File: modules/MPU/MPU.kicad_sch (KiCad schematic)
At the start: 6 parts, among them J1 CardConnector, U1 74HCT541, U2 74HCT00

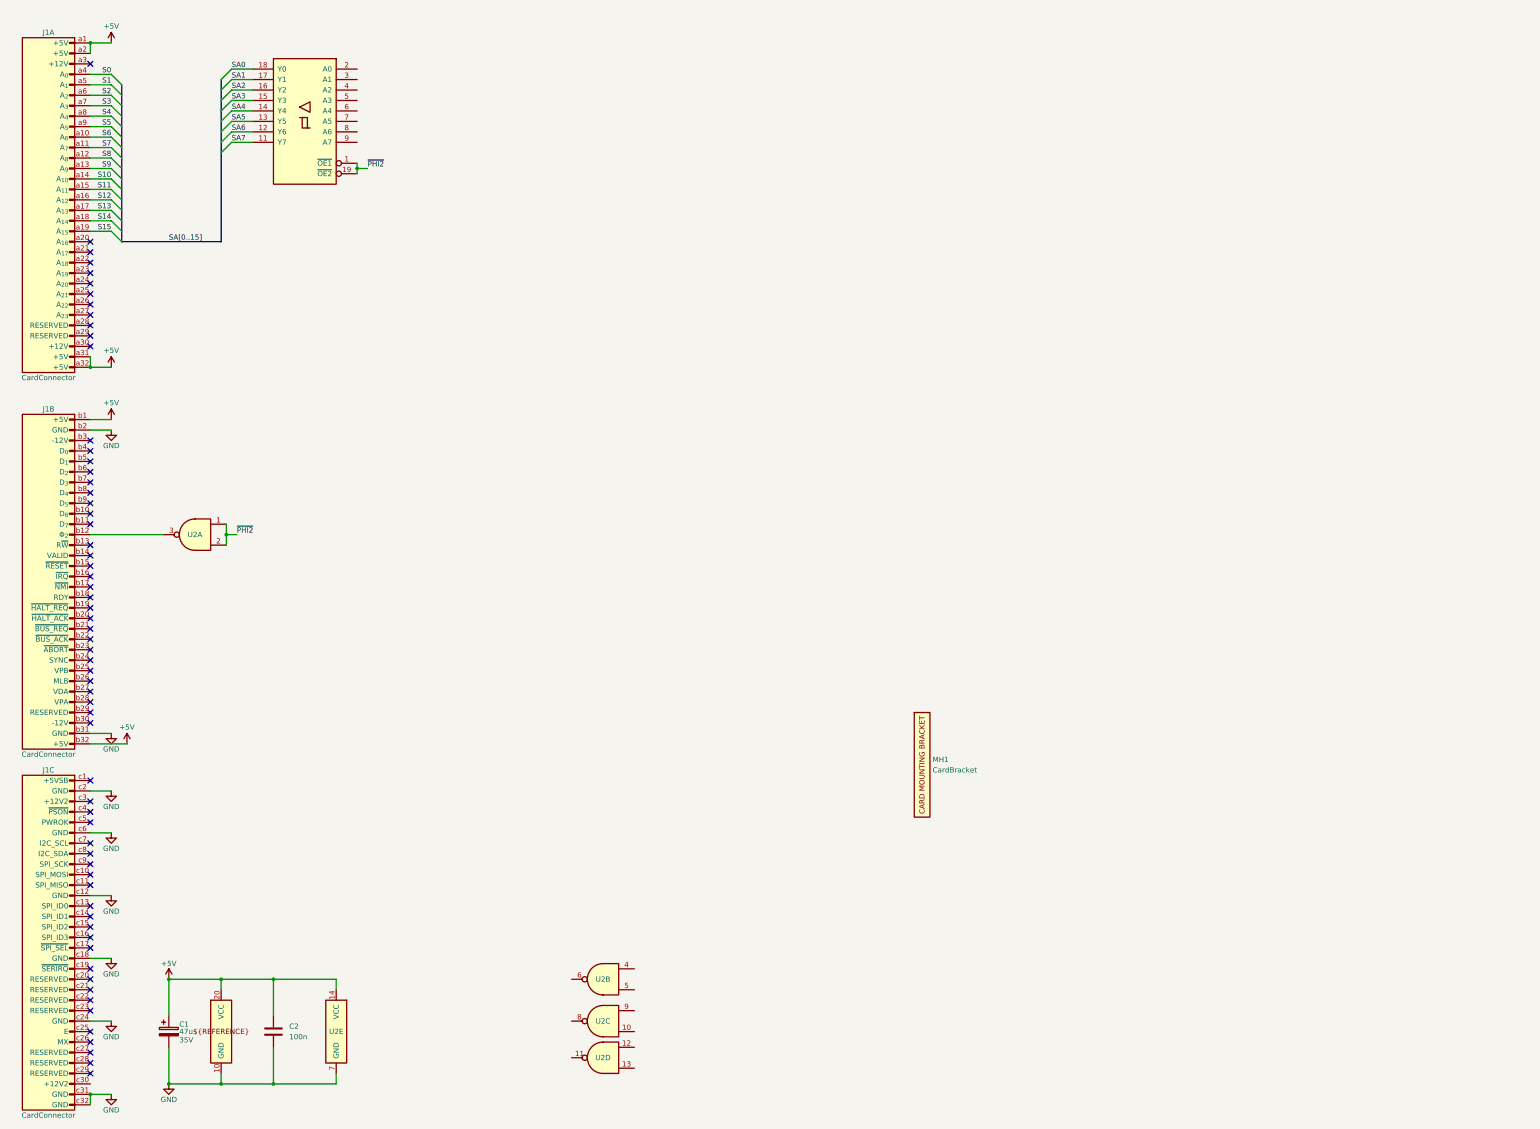
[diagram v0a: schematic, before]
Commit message: mpu wip
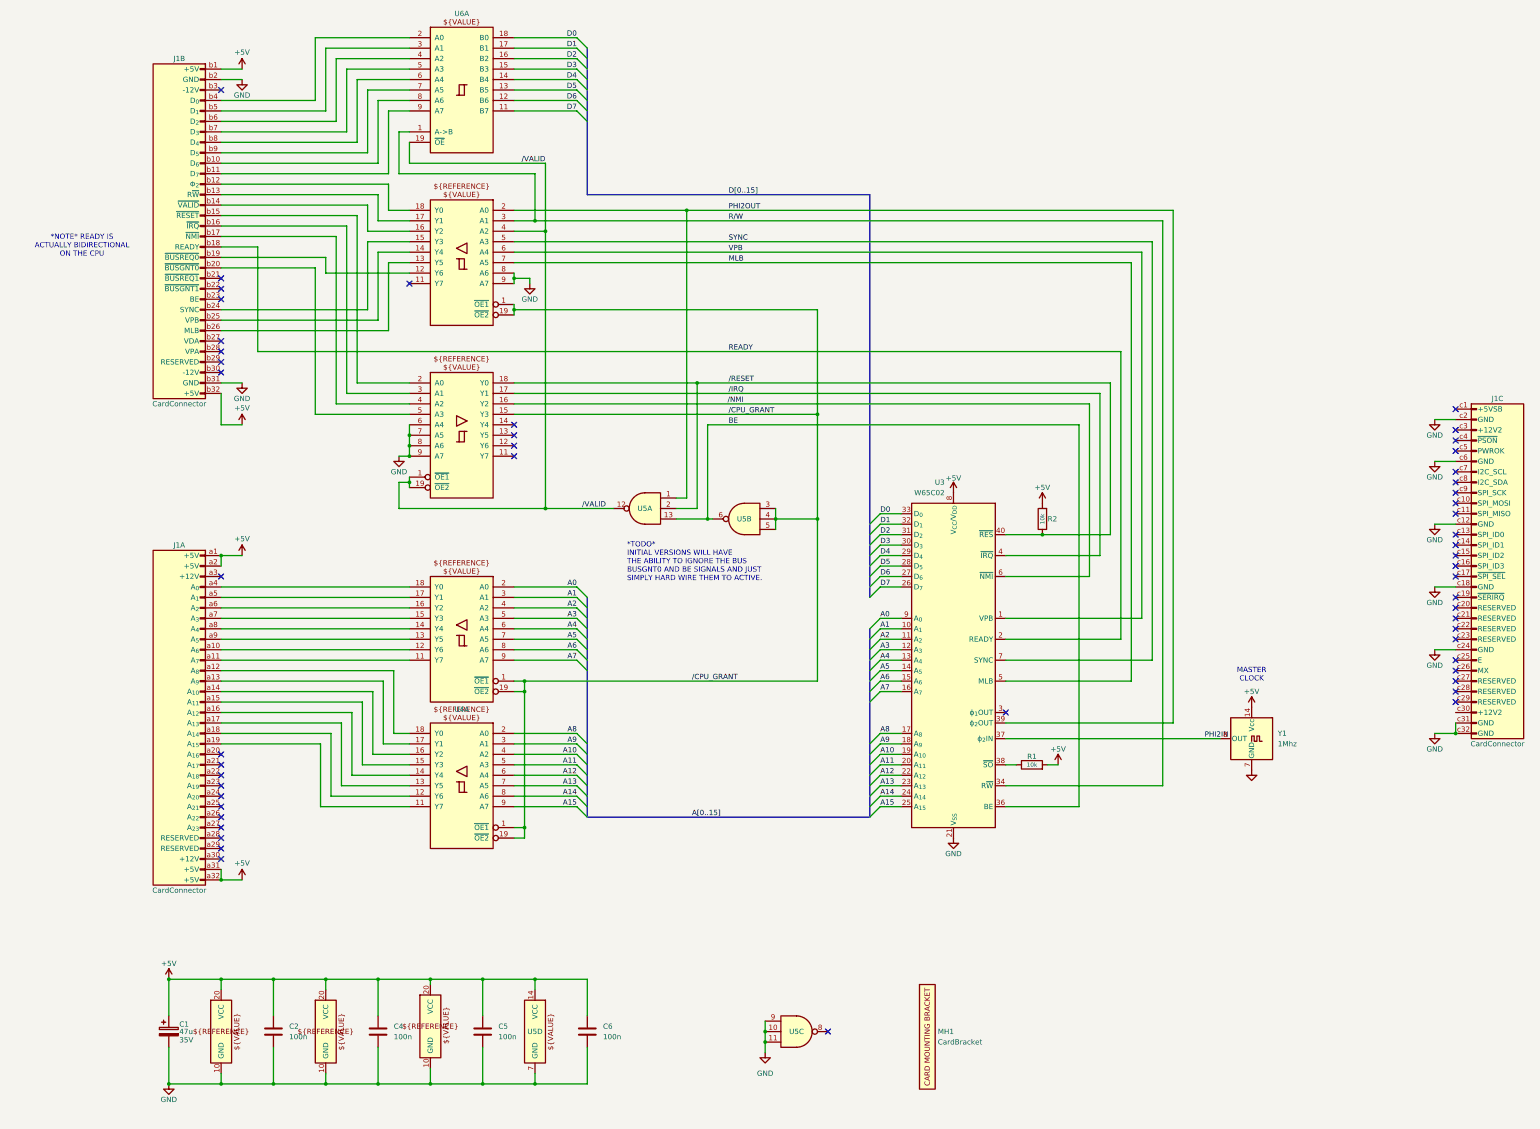
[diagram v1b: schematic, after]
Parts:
- removed U2: 74HCT00, IMNOTWOPR:DIP-14N, symbol IMNOTWOPR:74HCT00
- added C4, C5, C6: 100n, FormantKO:C_Rect_P200mil, symbol FormantKO:C
- added R1, R2: 10k, IMNOTWOPR:R_Axial_DIN0207_P400mil, symbol IMNOTWOPR:R
- added unit 1 of U1
- added U3: W65C02, IMNOTWOPR:DIP-40W, symbol IMNOTWOPR:W65C02
- added U4, U7, U8: 74HCT541, IMNOTWOPR:DIP-20N, symbol IMNOTWOPR:74HCT541
- added U5: 74HCT10, symbol IMNOTWOPR:74HCT10
- added U6: 74HCT245N, IMNOTWOPR:DIP-20N, symbol IMNOTWOPR:74HCT245
- added Y1: 1Mhz, Oscillator:Oscillator_DIP-14, symbol Oscillator:ACO-xxxMHz
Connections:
- net +5V: now also C4.1, C5.1, C6.1, R1.2, R2.2, U3.8 (V_{CC}/V_{DD}), U4.20 (VCC), U5.14 (VCC), U6.20 (VCC), Y1.14 (Vcc)
- net GND: now also C4.2, C5.2, C6.2, U3.21 (V_{SS}), U4.10 (GND), U5.10, U5.11, U5.7 (GND), U5.9, U6.10 (GND), U7.8 (A6), U7.9 (A7), U8.6 (A4), U8.7 (A5), U8.8 (A6), U8.9 (A7), Y1.7 (GND)
- net at J1.b12 (Φ_{2}): now also U7.18 (Y0)
- net at J1.b10 (D_{6}): now also U6.8 (A6)
- net at J1.b11 (D_{7}): now also U6.9 (A7)
- net at J1.b13 (R~{W}): now also U7.17 (Y1)
- net at J1.b14 (~{VALID}): now also U7.16 (Y2)
- net at J1.b15 (~{RESET}): now also U8.2 (A0)
- net at J1.b16 (~{IRQ}): now also U8.3 (A1)
- net at J1.b17 (~{NMI}): now also U8.4 (A2)
- net READY: now reaches J1.b18 (READY)
- net READY: now also U3.2 (READY)
- net at J1.b19 (~{BUSREQ0}): now also U7.12 (Y6)
- net at J1.b20 (~{BUSGNT0}): now also U8.5 (A3)
- net at J1.b24 (SYNC): now also U7.15 (Y3)
- net at J1.b25 (VPB): now also U7.14 (Y4)
- net at J1.b26 (MLB): now also U7.13 (Y5)
- net at J1.b4 (D_{0}): now also U6.2 (A0)
- net at J1.b5 (D_{1}): now also U6.3 (A1)
- net at J1.b6 (D_{2}): now also U6.4 (A2)
- net at J1.b7 (D_{3}): now also U6.5 (A3)
- net at J1.b8 (D_{4}): now also U6.6 (A4)
- net at J1.b9 (D_{5}): now also U6.7 (A5)
- net S0: no longer names the net of J1.a4 (A_{0})
- net S0: now also U1.18 (Y0)
- net S1: no longer names the net of J1.a5 (A_{1})
- net S1: now also U1.17 (Y1)
- net S10: no longer names the net of J1.a14 (A_{10})
- net S10: now also U4.16 (Y2)
- net S11: no longer names the net of J1.a15 (A_{11})
- net S11: now also U4.15 (Y3)
- net S12: no longer names the net of J1.a16 (A_{12})
- net S12: now also U4.14 (Y4)
- net S13: no longer names the net of J1.a17 (A_{13})
- net S13: now also U4.13 (Y5)
- net S14: no longer names the net of J1.a18 (A_{14})
- net S14: now also U4.12 (Y6)
- net S15: no longer names the net of J1.a19 (A_{15})
- net S15: now also U4.11 (Y7)
- net S2: no longer names the net of J1.a6 (A_{2})
- net S2: now also U1.16 (Y2)
- net S3: no longer names the net of J1.a7 (A_{3})
- net S3: now also U1.15 (Y3)
- net S4: no longer names the net of J1.a8 (A_{4})
- net S4: now also U1.14 (Y4)
- net S5: no longer names the net of J1.a9 (A_{5})
- net S5: now also U1.13 (Y5)
- net S6: no longer names the net of J1.a10 (A_{6})
- net S6: now also U1.12 (Y6)
- net S7: no longer names the net of J1.a11 (A_{7})
- net S7: now also U1.11 (Y7)
- net S8: no longer names the net of J1.a12 (A_{8})
- net S8: now also U4.18 (Y0)
- net S9: no longer names the net of J1.a13 (A_{9})
- net S9: now also U4.17 (Y1)
- removed net SA0: U1.18 (Y0)
- removed net SA1: U1.17 (Y1)
- removed net SA2: U1.16 (Y2)
- removed net SA3: U1.15 (Y3)
- removed net SA4: U1.14 (Y4)
- removed net SA5: U1.13 (Y5)
- removed net SA6: U1.12 (Y6)
- removed net SA7: U1.11 (Y7)
- removed net ~{PHI2}: U1.1 (~{OE1}), U1.19 (~{OE2})
- new net: R1.1, U3.38 (~{SO})
- new net A0: U1.2 (A0), U3.9 (A_{0})
- new net A1: U1.3 (A1), U3.10 (A_{1})
- new net A10: U3.19 (A_{10}), U4.4 (A2)
- new net A11: U3.20 (A_{11}), U4.5 (A3)
- new net A12: U3.22 (A_{12}), U4.6 (A4)
- new net A13: U3.23 (A_{13}), U4.7 (A5)
- new net A14: U3.24 (A_{14}), U4.8 (A6)
- new net A15: U3.25 (A_{15}), U4.9 (A7)
- new net A2: U1.4 (A2), U3.11 (A_{2})
- new net A3: U1.5 (A3), U3.12 (A_{3})
- new net A4: U1.6 (A4), U3.13 (A_{4})
- new net A5: U1.7 (A5), U3.14 (A_{5})
- new net A6: U1.8 (A6), U3.15 (A_{6})
- new net A7: U1.9 (A7), U3.16 (A_{7})
- new net A8: U3.17 (A_{8}), U4.2 (A0)
- new net A9: U3.18 (A_{9}), U4.3 (A1)
- new net BE: U3.36 (BE), U5.13, U5.6
- new net D0: U3.33 (D_{0}), U6.18 (B0)
- new net D1: U3.32 (D_{1}), U6.17 (B1)
- new net D2: U3.31 (D_{2}), U6.16 (B2)
- new net D3: U3.30 (D_{3}), U6.15 (B3)
- new net D4: U3.29 (D_{4}), U6.14 (B4)
- new net D5: U3.28 (D_{5}), U6.13 (B5)
- new net D6: U3.27 (D_{6}), U6.12 (B6)
- new net D7: U3.26 (D_{7}), U6.11 (B7)
- new net MLB: U3.5 (MLB), U7.7 (A5)
- new net PHI2IN: U3.37 (ϕ_{2}IN), Y1.8 (OUT)
- new net PHI2OUT: U3.39 (ϕ_{2}OUT), U5.1, U7.2 (A0)
- new net R/W: U3.34 (R~{W}), U6.1 (A->B), U7.3 (A1)
- new net SYNC: U3.7 (SYNC), U7.5 (A3)
- new net VPB: U3.1 (VPB), U7.6 (A4)
- new net /CPU_GRANT: U1.1 (~{OE1}), U1.19 (~{OE2}), U4.1 (~{OE1}), U4.19 (~{OE2}), U5.3, U5.4, U5.5, U7.1 (~{OE1}), U7.19 (~{OE2}), U8.15 (Y3)
- new net /IRQ: U3.4 (~{IRQ}), U8.17 (Y1)
- new net /NMI: U3.6 (~{NMI}), U8.16 (Y2)
- new net /RESET: R2.1, U3.40 (~{RES}), U5.2, U8.18 (Y0)
- new net /VALID: U5.12, U6.19 (~{OE}), U7.4 (A2), U8.1 (~{OE1}), U8.19 (~{OE2})
- no-connect marks 63 -> 51
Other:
- note added: "*NOTE* READY IS ACTUALLY BIDIRECTIONAL ON THE CPU"
- note added: "*TODO* INITIAL VERSIONS WILL HAVE THE ABILITY TO IGNORE THE BUS BUSGNT0 AND BE SIGNALS AND JUST SIMPLY HARD WIRE THEM TO ACTIVE."
- note added: "MASTER CLOCK"
- moved on the sheet: J1A, J1B, J1C, MH1
